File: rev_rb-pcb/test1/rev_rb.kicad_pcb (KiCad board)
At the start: 2 copper layers, 65.9 x 84.5 mm, 60 parts, among them CON1 BARREL_JACK, J1 audio-jack, P1 CONN_01X03, P2 CONN_01X03, Q1 MOSFET-PCHANNELSMD, Q2 MOSFET-NCHANNELSMD, U1 STM32F103RB, U2 PC817, U3 PC817, U4 PC817, U6 10-XX_B3F-10XX, U7 MIC5219BM5_SOT23-5, U8 XC63FPM_SOT23, Y1 8Mhz

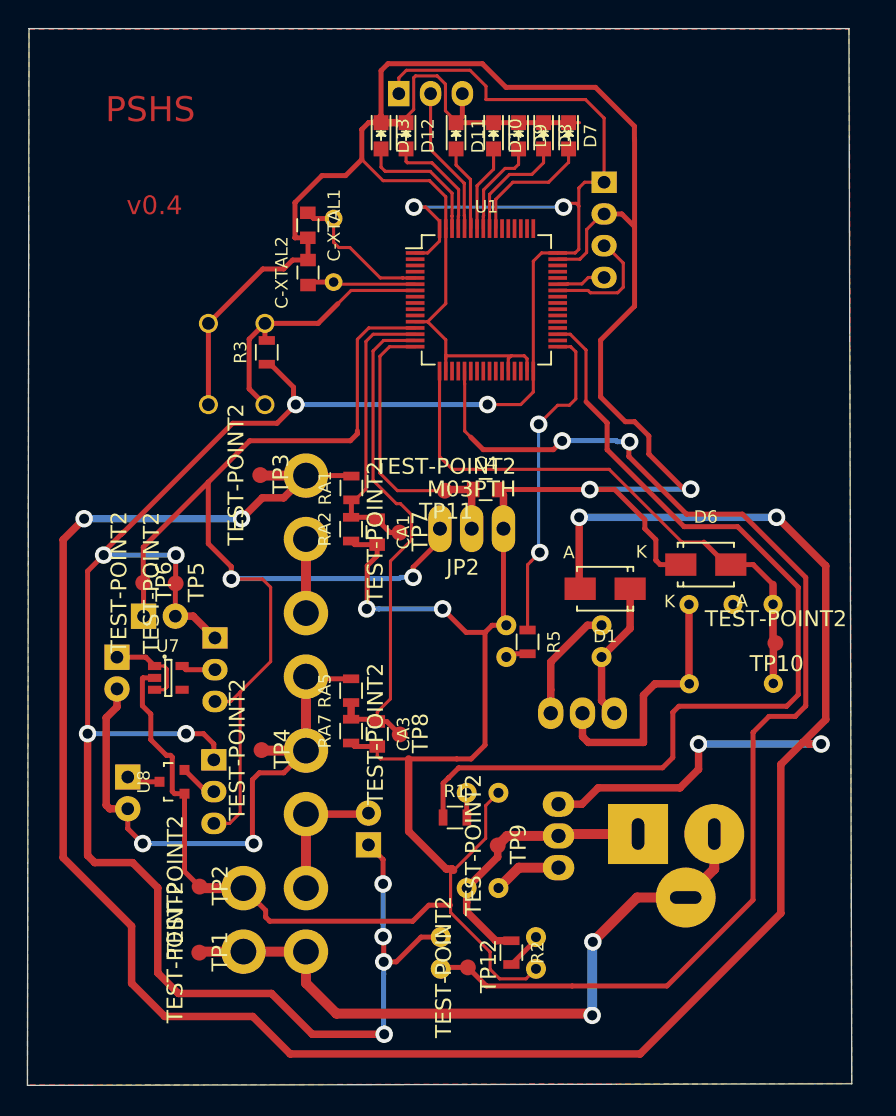
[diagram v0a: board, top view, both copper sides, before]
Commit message: try again
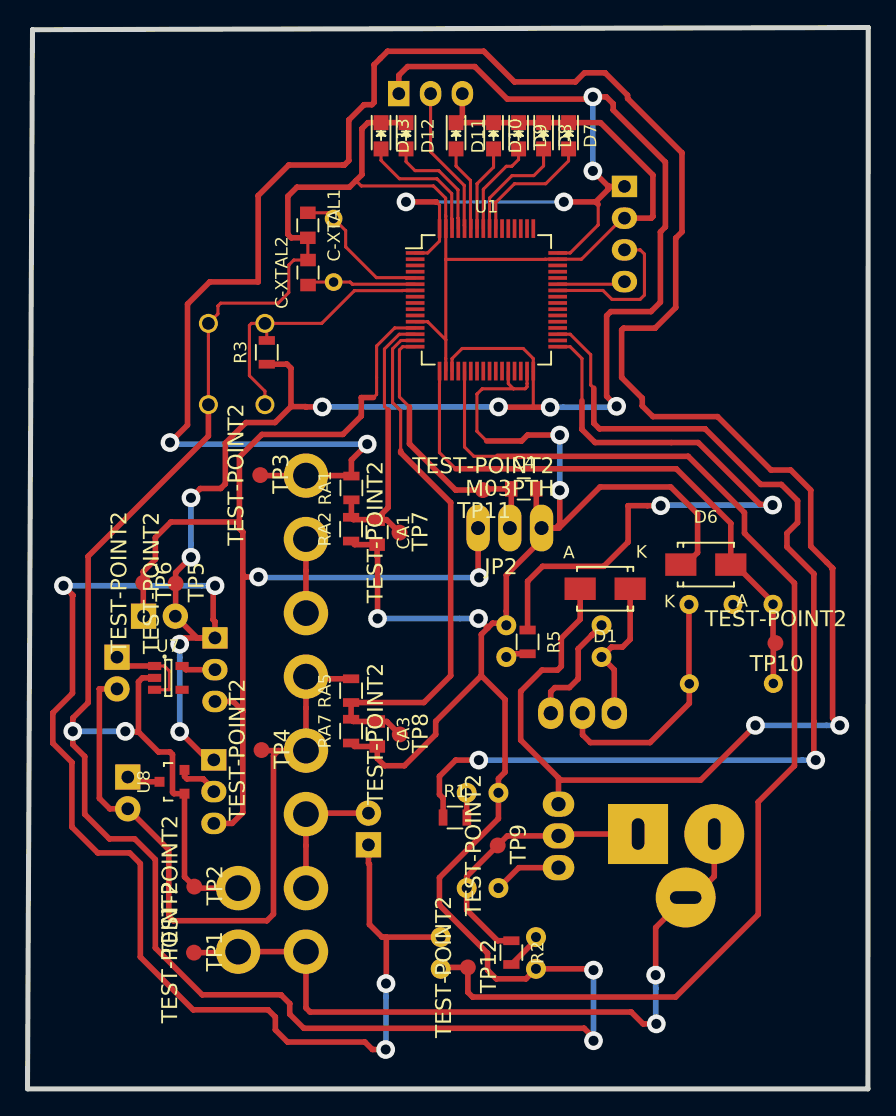
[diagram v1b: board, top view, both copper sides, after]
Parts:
- moved C4 3.05 mm to (128.3, 96.4)
- moved JP2 3.05 mm to (124.6, 99.5)
- moved TP11 3.05 mm to (125.0, 96.4)
- moved P-COMM1 1.66 mm to (136.3, 72.2)
- moved JP1 0.42 mm to (105.4, 130.8)
- moved TP1 0.42 mm to (101.9, 133.5)
- moved TP2 0.42 mm to (101.9, 128.2)
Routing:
- net VDD: track 216.8 -> 270.8 mm, vias 12 -> 16
- net GND: track 313.9 -> 362.8 mm, vias 4 -> 8
- net /CON-LAMP: track 26.1 -> 53.5 mm
- net +6V: track 47.2 -> 57.9 mm, vias 2 -> 0
- net /CON-PV: track 76.1 -> 83.9 mm, vias 0 -> 2
- net +BATT: track 207.6 -> 203.8 mm, vias 6 -> 4
- net GNDPWR: track 55.9 -> 59.5 mm
- net /ADC-BATT2: track 41.7 -> 44.7 mm
- net Net-(P-COMM1-Pad3): track 9.55 -> 12.4 mm
- net +3V3: track 94.1 -> 92.2 mm
- net /ADC-DIM: track 23.7 -> 22.1 mm
- net Net-(P-COMM1-Pad4): track 3.94 -> 5.43 mm
- net Net-(J1-Pad2): track 21.1 -> 19.7 mm
- net /ADC-LAMP: track 45.8 -> 46.7 mm
- net /NRST: track 22.1 -> 22.7 mm
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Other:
- board size 65.9 x 84.5 mm -> 67.2 x 84.9 mm
- board text removed: "PSHS"
- board text removed: "v0.4"

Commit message: progress
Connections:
- net Net-(P-COMM1-Pad3) renamed /TX
- net Net-(P-COMM1-Pad4) renamed /RX
